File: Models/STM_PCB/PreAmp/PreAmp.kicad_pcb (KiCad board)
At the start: 2 copper layers, 18.9 x 16.5 mm, 7 parts, among them J1 Conn_Coaxial, J2 Conn_01x03_Socket, J3 Conn_01x03_Socket, U1 AD8615

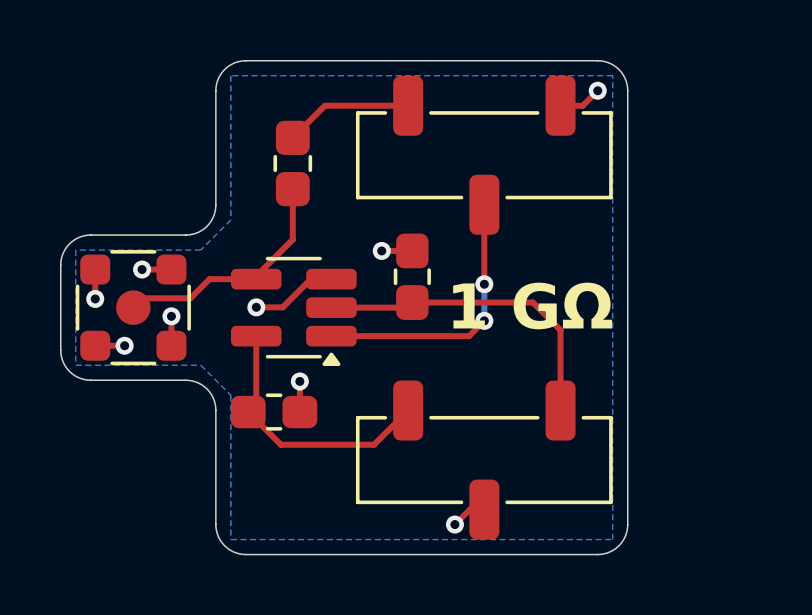
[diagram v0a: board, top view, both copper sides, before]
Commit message: Fixed the PCB
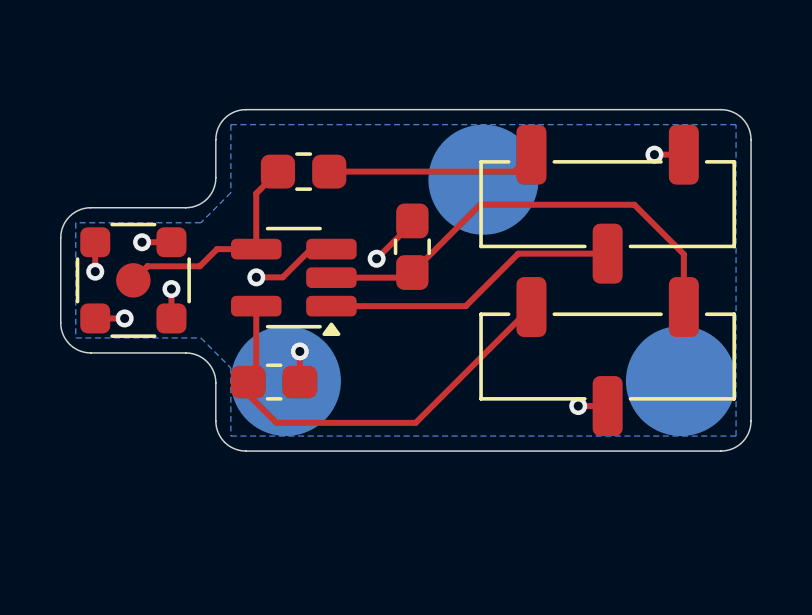
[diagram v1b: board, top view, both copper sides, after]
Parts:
- added H1: MountingHole_Pad, Connector_Custom:KJ_D21SH, B.Cu at (159.8, 101.5)
- added H2: MountingHole_Pad, Connector_Custom:KJ_D21SH, B.Cu at (166.3, 94.8)
- added H3: MountingHole_Pad, Connector_Custom:KJ_D21SH, B.Cu at (172.9, 101.5)
- C1, C2: value 1 uF, 0603 -> 1 uF, 0603, 25V, X7R
- moved J2 5.37 mm to (170.5, 100.7)
- moved J3 4.42 mm to (170.5, 95.6)
- moved C1 1.00 mm to (159.4, 101.5)
- moved C2 1.00 mm to (164.0, 97.0)
- moved U1 1.00 mm to (160.0, 98.1)
- moved J1 0.91 mm to (154.7, 98.2)
- moved R1 0.45 mm to (160.3, 94.5), turned to 0 degrees
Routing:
- net /2.5V: track 8.89 -> 14.5 mm
- net /-1.5V: track 10.8 -> 15.2 mm
- net /PreVoltage: track 4.29 -> 6.97 mm
- net /AD8615_Output: track 9.18 -> 9.93 mm, vias 2 -> 0
- net /Current: track 8.00 -> 7.41 mm
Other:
- board size 18.9 x 16.5 mm -> 23 x 11.4 mm
- board text removed: "1 GΩ"
- board text removed: "Rearrange this board to be thinner in the Y dimension"
